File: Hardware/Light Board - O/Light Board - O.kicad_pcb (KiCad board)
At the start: 2 copper layers, 46.8 x 36.8 mm, 11 parts, among them J1 V+, J2 V-

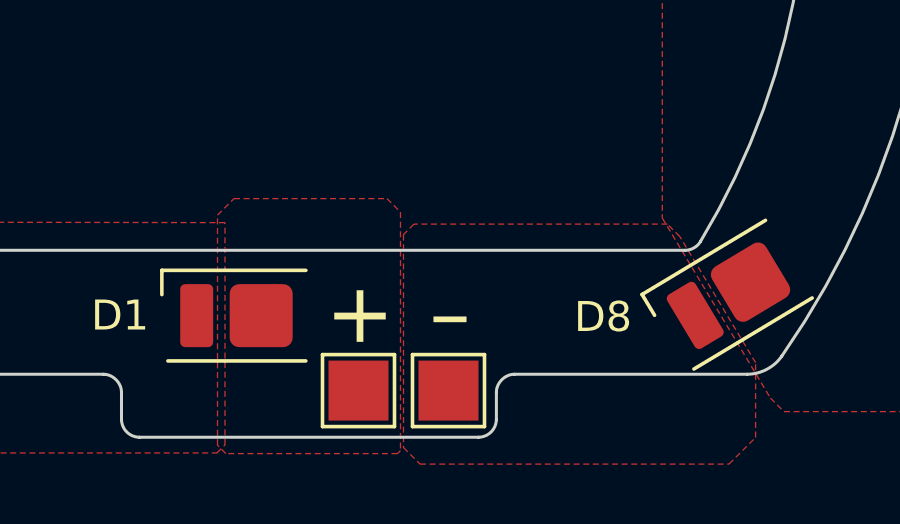
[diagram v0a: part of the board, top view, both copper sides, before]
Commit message: Finished all light boards
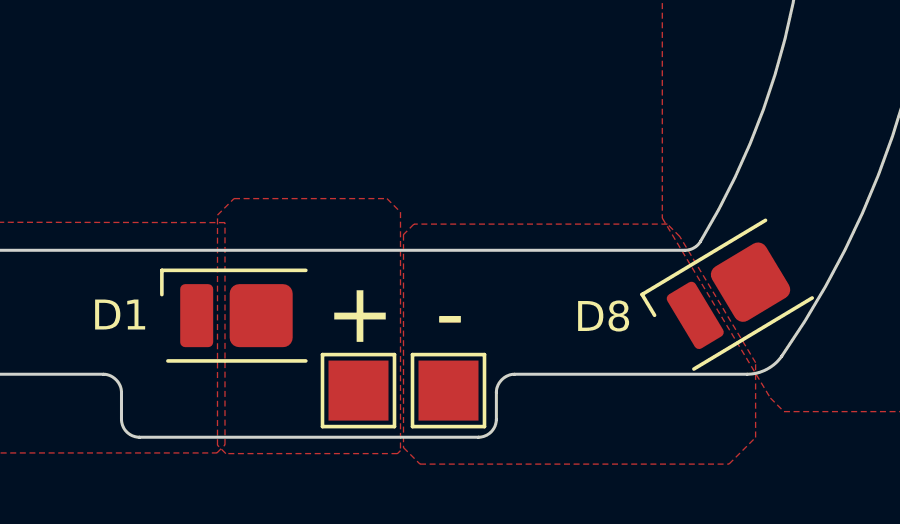
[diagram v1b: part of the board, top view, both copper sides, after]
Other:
- board text added: "-"
- board text removed: "–"
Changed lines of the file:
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@@
 		)
 	)
-	(gr_text "–"
+	(gr_text "-"
 		(at 145.1 112.1 0)
 		(layer "F.SilkS")
